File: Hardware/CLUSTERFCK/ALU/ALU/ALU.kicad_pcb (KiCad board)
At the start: 2 copper layers, 119 x 96 mm, 33 parts, among them J1 Conn_02x08_Counter_Clockwise, J2 Conn_02x08_Counter_Clockwise, J3 Conn_02x08_Counter_Clockwise, U1 74LS86, U2 74LS283, U3 74LS283, U4 74LS86, U5 74LS02, U6 74LS08

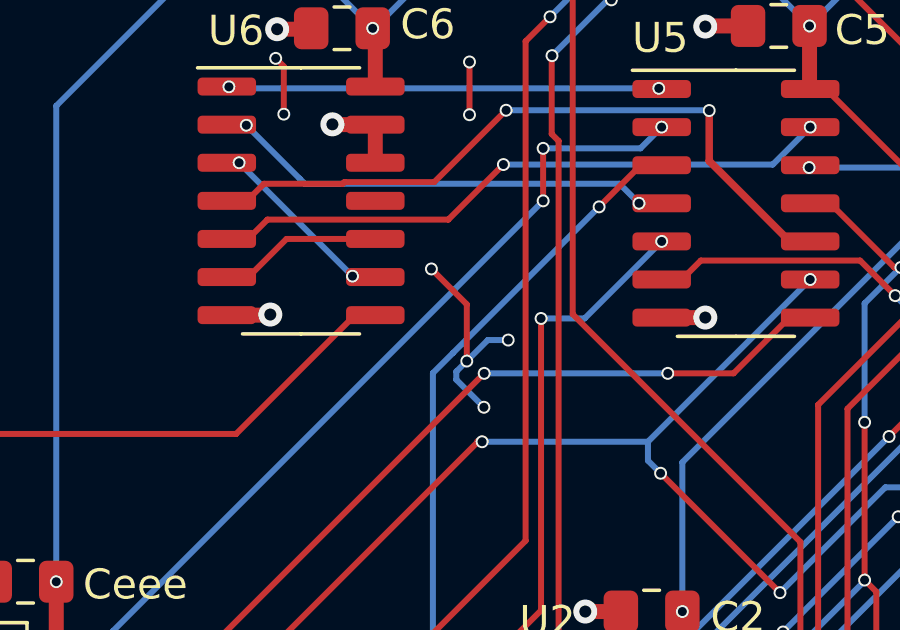
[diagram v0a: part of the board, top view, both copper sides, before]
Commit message: 0050 | 5h | Ram module
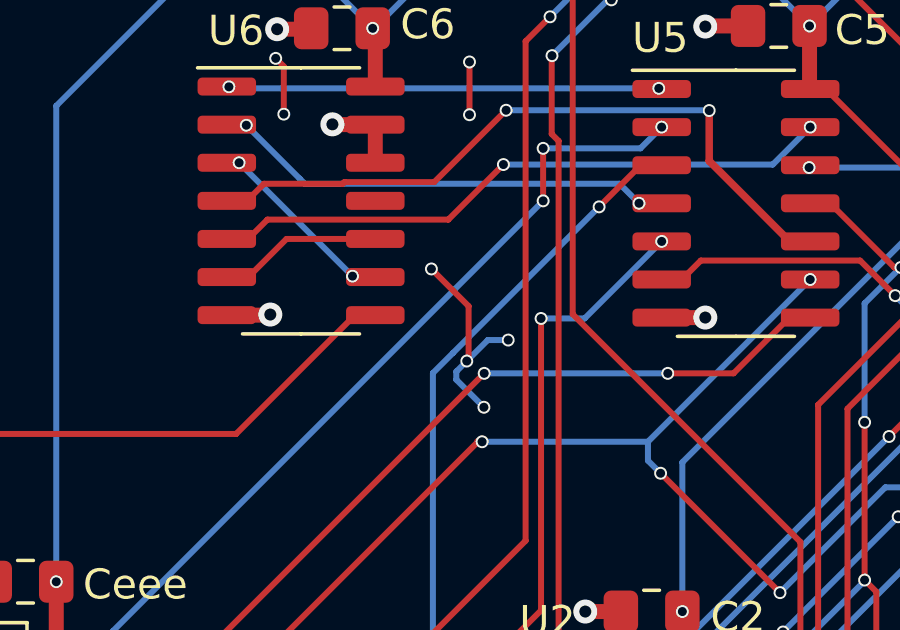
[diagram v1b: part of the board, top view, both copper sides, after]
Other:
- net class Default removed
